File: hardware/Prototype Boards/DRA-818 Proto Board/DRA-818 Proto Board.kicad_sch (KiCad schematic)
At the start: 36 parts, among them J1 VCC, J2 UART, J3 AUDIO, J4 GPIO, K1 TLP241A, Q1 DMN67D8LW-13, Q2 BSS138, Q3 BSS138, Q4 Q_NPN_BCE, SW1 H/L_DIP_SW

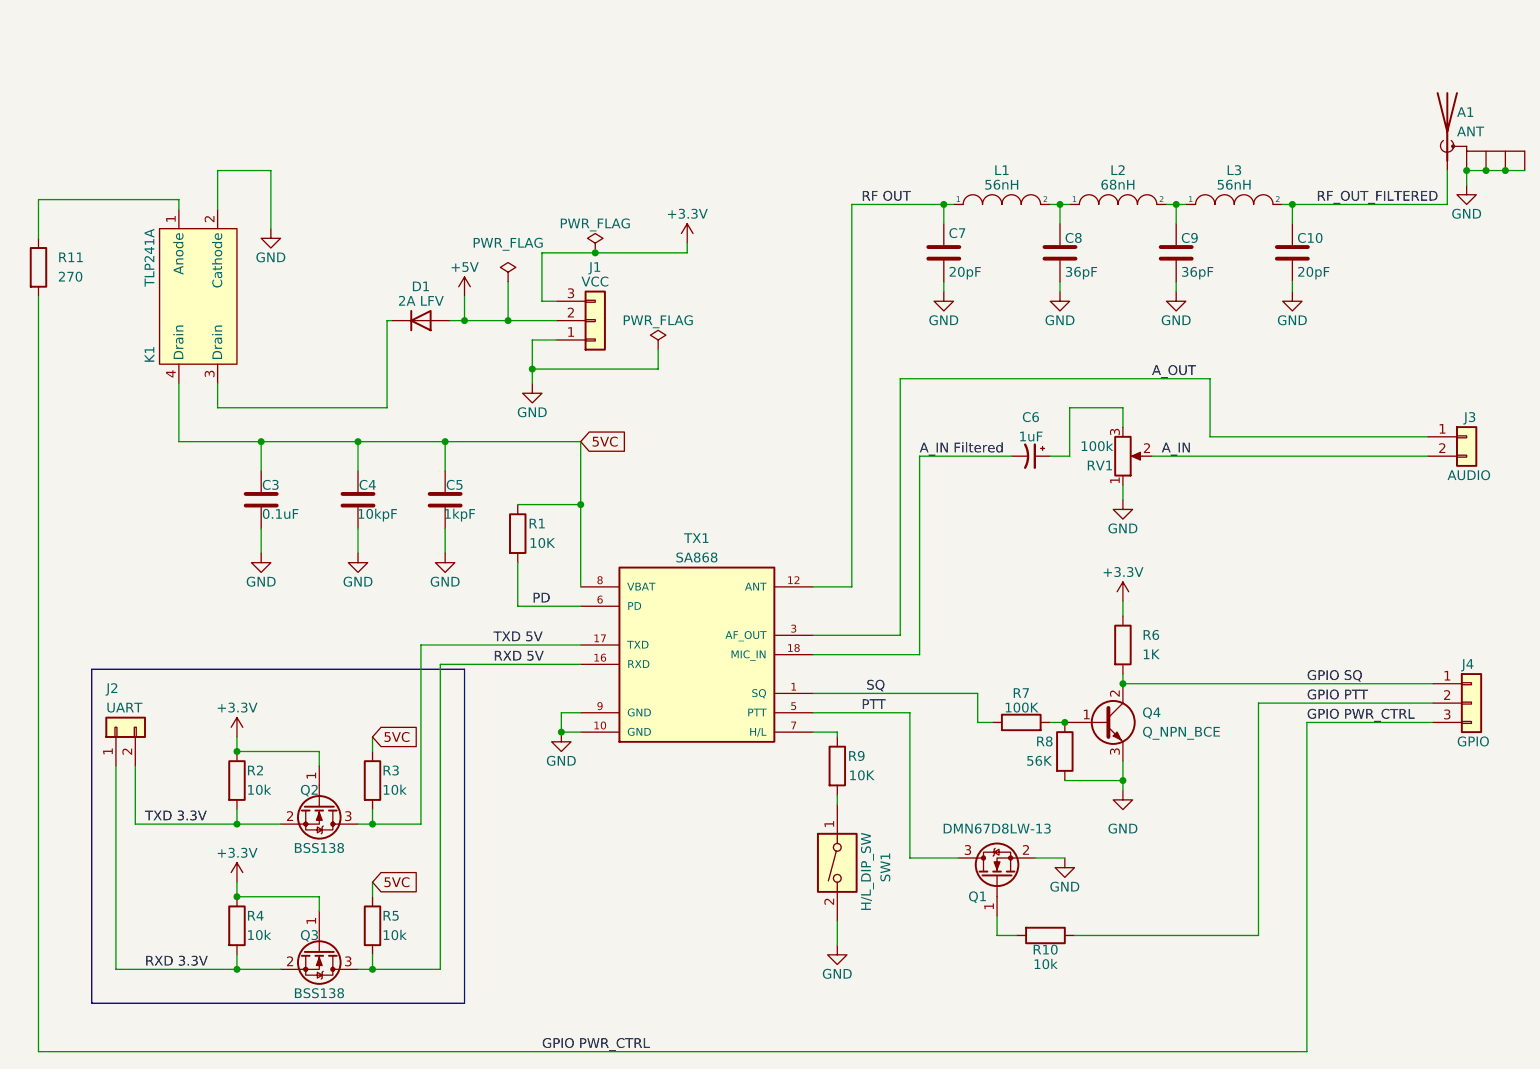
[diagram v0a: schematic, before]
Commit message: hardware and latex updates
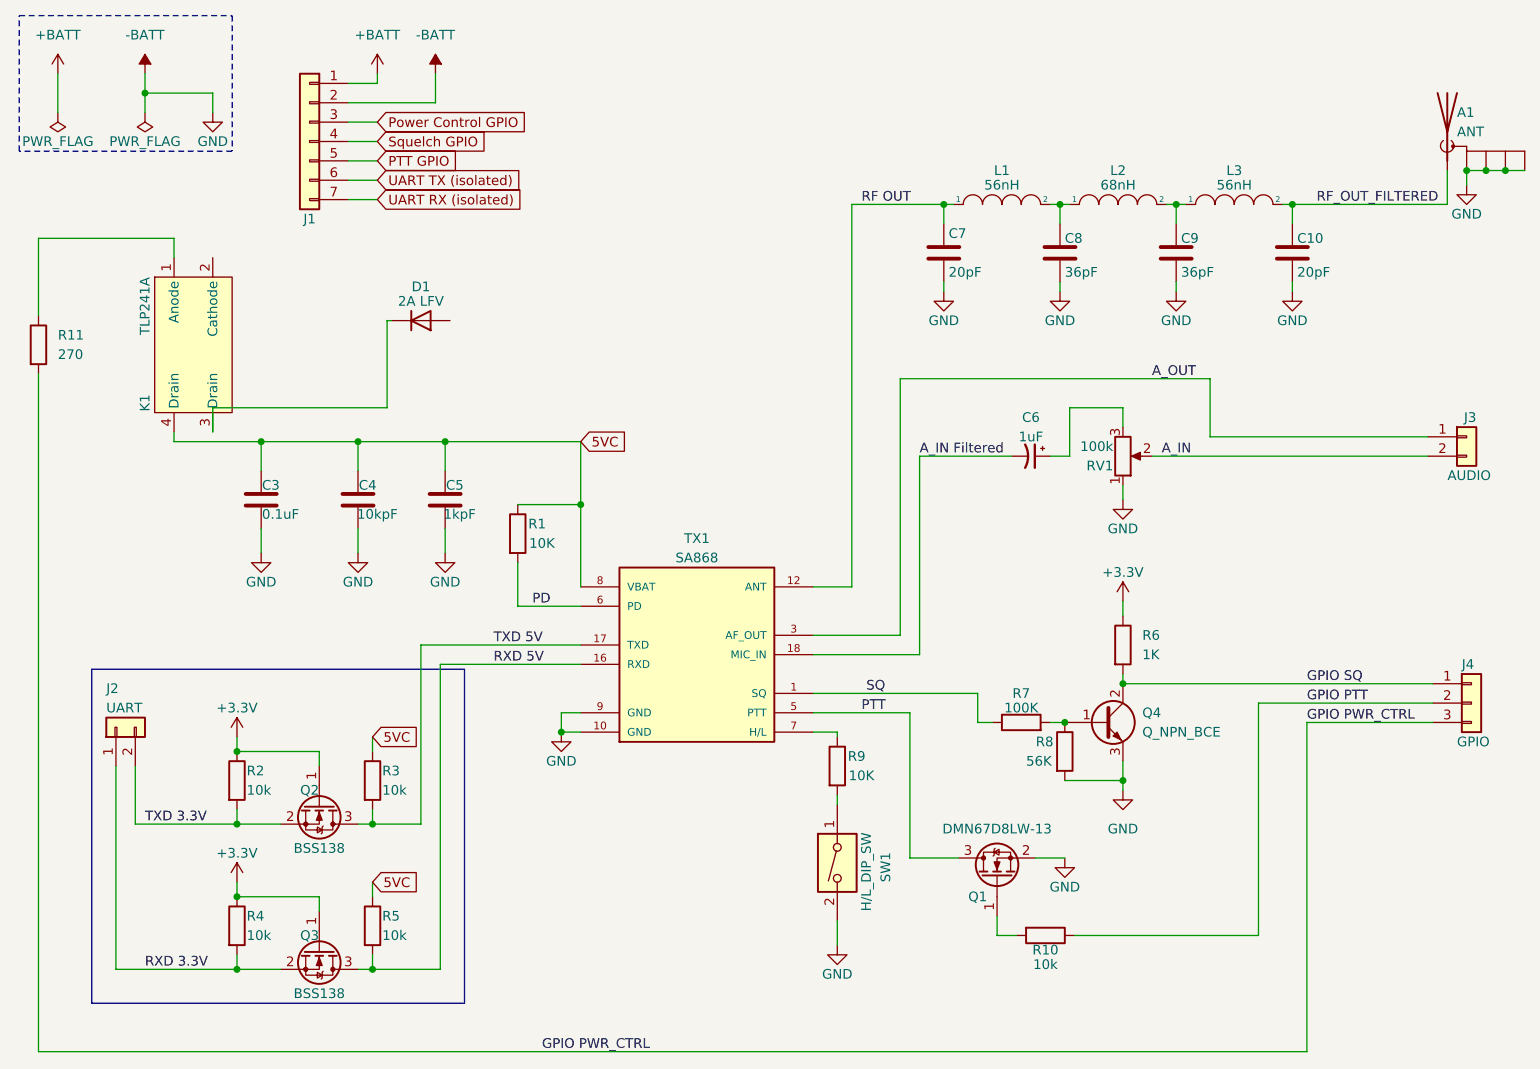
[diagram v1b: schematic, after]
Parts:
- removed J1: VCC, Connector_PinHeader_2.54mm:PinHeader_1x03_P2.54mm_Vertical, symbol Connector_Generic:Conn_01x03
- added J1: ~, Connector_PinHeader_2.54mm:PinHeader_1x03_P2.54mm_Vertical, symbol Connector_Generic:Conn_01x07
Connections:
- net +5V: no longer names the net of D1.2 (A)
- net GND renamed -BATT
- net -BATT: now also J1.2 (Pin_2); no longer K1.2 (Cathode)
- new net +BATT: J1.1 (Pin_1)
- new net PTT GPIO: J1.5 (Pin_5)
- new net Power Control GPIO: J1.3 (Pin_3)
- new net Squelch GPIO: J1.4 (Pin_4)
- new net UART RX (isolated): J1.7 (Pin_7)
- new net UART TX (isolated): J1.6 (Pin_6)
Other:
- moved on the sheet: K1, R11
